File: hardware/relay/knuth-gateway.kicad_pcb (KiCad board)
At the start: 2 copper layers, 65.4 x 57.1 mm, 12 parts, among them J1 Screw_Terminal_01x03, J2 Screw_Terminal_01x03, J3 FeatherLora1, J4 FeatherLora2, J5 Conn_01x07_Female, SW2 SW_SPDT

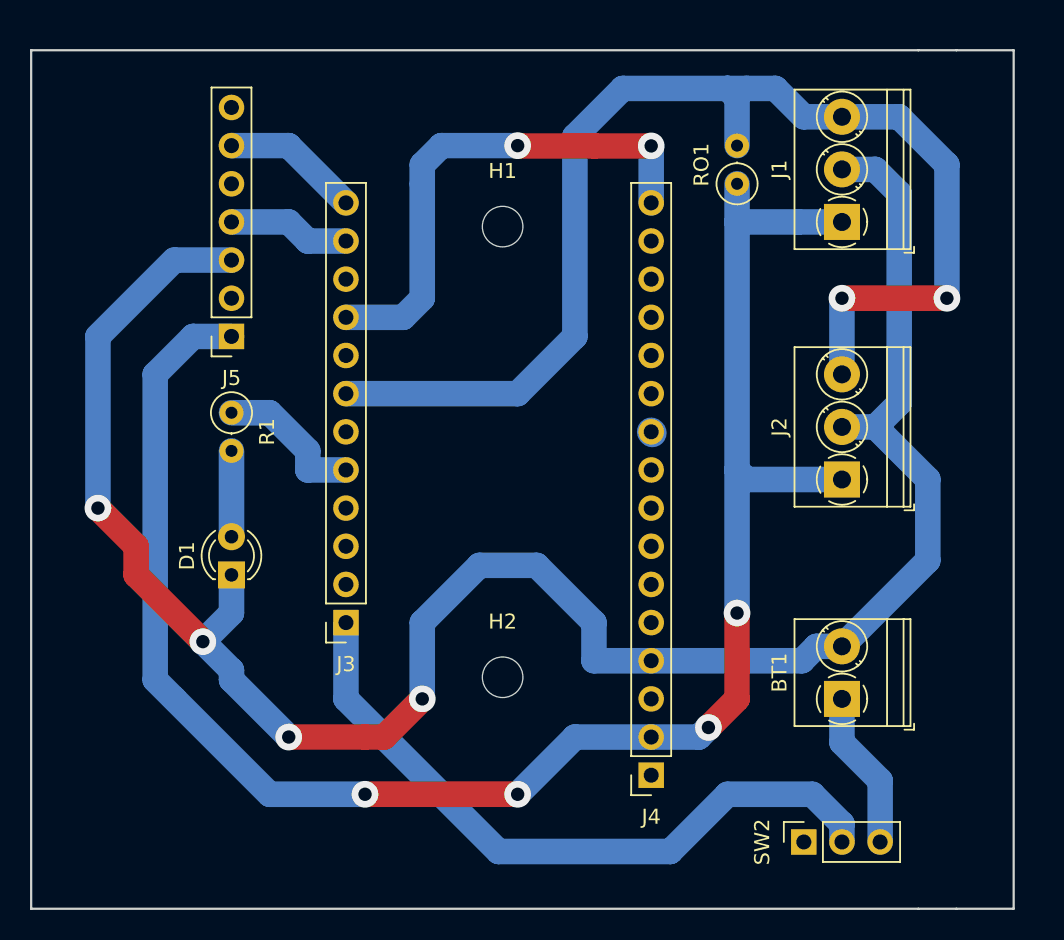
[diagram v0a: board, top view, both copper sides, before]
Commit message: update
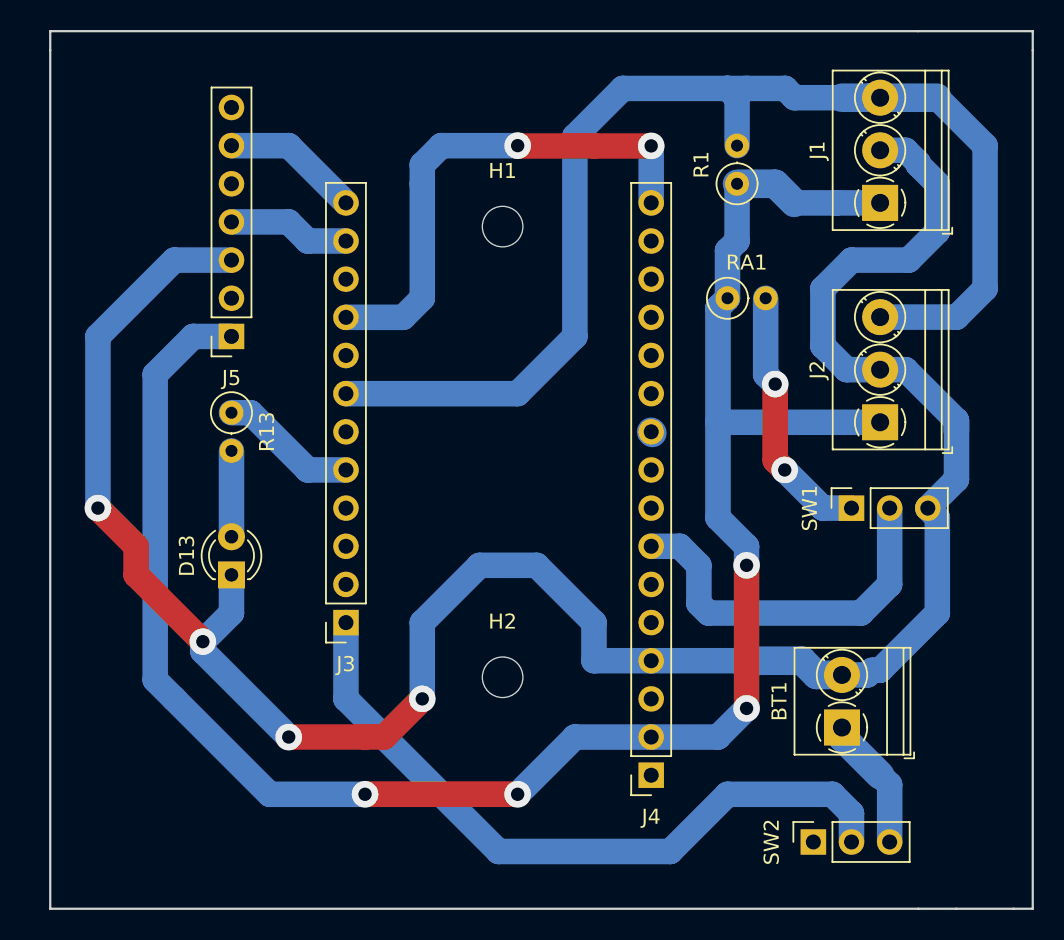
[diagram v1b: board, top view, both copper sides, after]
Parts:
- added RA1: R, Resistor_THT:R_Axial_DIN0207_L6.3mm_D2.5mm_P2.54mm_Vertical, F.Cu at (54.6, 19.1)
- added SW1: SW_SPDT, Connector_PinSocket_2.54mm:PinSocket_1x03_P2.54mm_Vertical, F.Cu at (62.9, 33.0)
- moved J2 4.58 mm to (64.8, 27.3)
- moved J1 2.84 mm to (64.8, 12.7)
- moved BT1 1.91 mm to (62.2, 47.6)
- moved SW2 0.64 mm to (60.3, 55.2)
- renumbered D1 to D13, RO1 to R1, R1 to R13
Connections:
- J4 pad 7: (no net) -> A2
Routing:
- net A2: track 0.00 -> 25.1 mm
- net Net-(RA1-Pad2): track 0.00 -> 17.5 mm, vias 0 -> 2
- net GND: track 138.5 -> 151.8 mm
- net +3V3: track 119.5 -> 128.4 mm
- net Net-(BT1-Pad1): track 10.6 -> 8.94 mm
- net D10: track 83.3 -> 81.7 mm, vias 2 -> 0
- net VBAT: track 45.9 -> 47.0 mm
- net D12: track 9.94 -> 9.20 mm
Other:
- board size 65.4 x 57.1 mm -> 65.4 x 58.4 mm
